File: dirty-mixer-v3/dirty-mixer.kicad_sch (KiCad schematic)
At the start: 10 parts, among them J1 AudioJack2_SwitchT, J2 AudioJack2_SwitchT, J3 AudioJack2_SwitchT, J4 AudioJack2_SwitchT, J5 AudioJack2_SwitchT, SW1 SW_SPDT, SW2 SW_SPDT

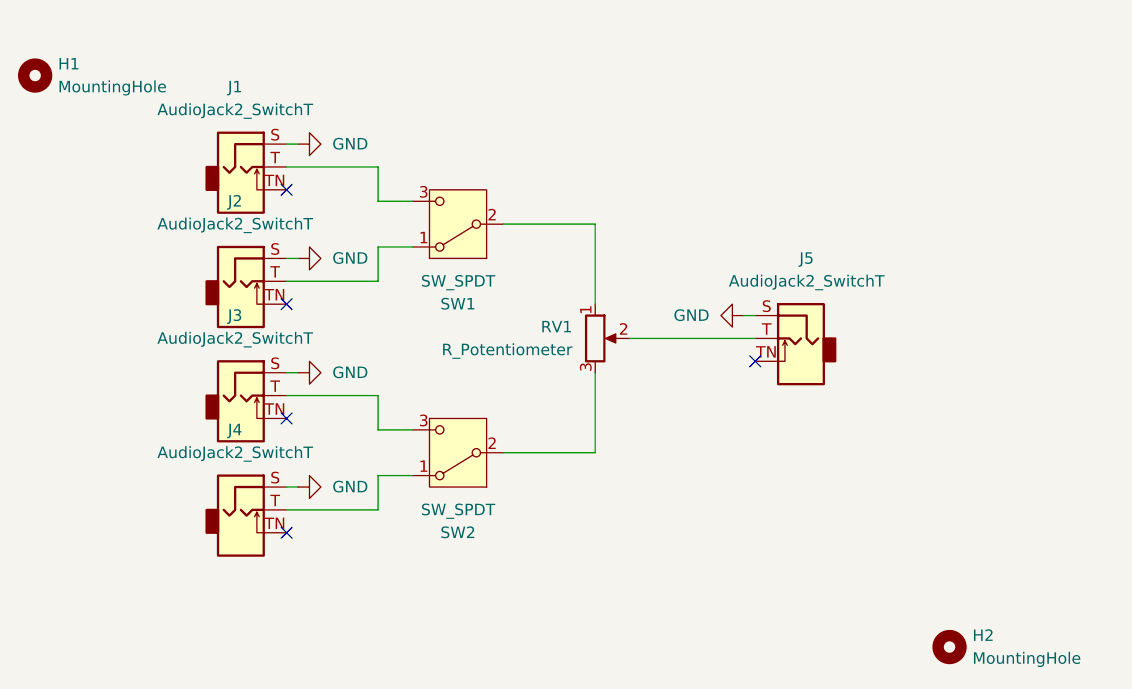
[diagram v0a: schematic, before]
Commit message: some pcb changes
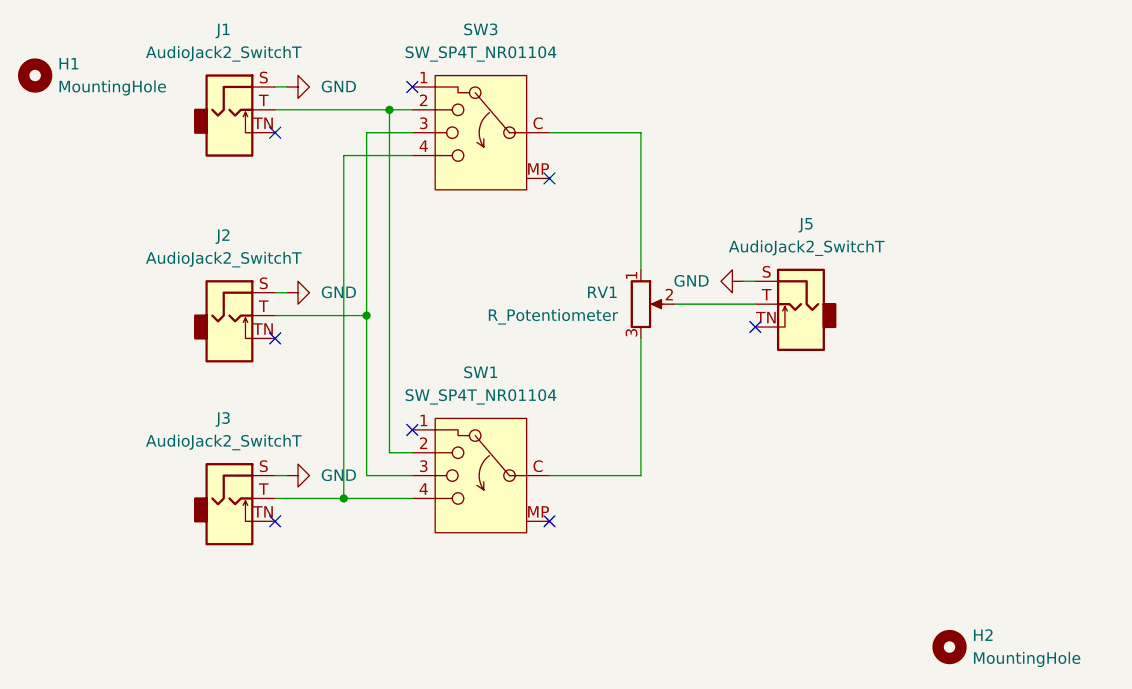
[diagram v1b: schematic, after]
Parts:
- removed J4: AudioJack2_SwitchT, Connector_Audio:Jack_3.5mm_QingPu_WQP-PJ398SM_Vertical_CircularHoles, symbol Connector_Audio:AudioJack2_SwitchT
- removed SW1, SW2: SW_SPDT, Custom:ANT13SEC_CRS, symbol Switch:SW_SPDT
- added SW1, SW3: SW_SP4T_NR01104, Button_Switch_THT:SW_NKK_NR01, symbol Switch:SW_SP4T_NR01104
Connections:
- net at J3.T: now also SW1.4, SW3.4
- net at RV1.1: now also SW3.C (Common)
- net at RV1.3: now also SW1.C (Common)
- net at J1.T: now also SW1.2, SW3.2
- net at J2.T: now also SW1.3, SW3.3
- no-connect marks 5 -> 8
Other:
- moved on the sheet: J1, J2, J3, J5, RV1
